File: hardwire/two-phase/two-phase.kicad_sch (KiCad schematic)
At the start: 75 parts, among them Q1 BC847, Q2 IRF3205, Q3 IRF3205, Q4 IRF3205, Q5 IRF3205, U1 74HC244, U2 UC2845_SOIC8, U3 IRS2003, U4 IRS2003, U5 LM7812_TO220, U6 LM7805_TO220

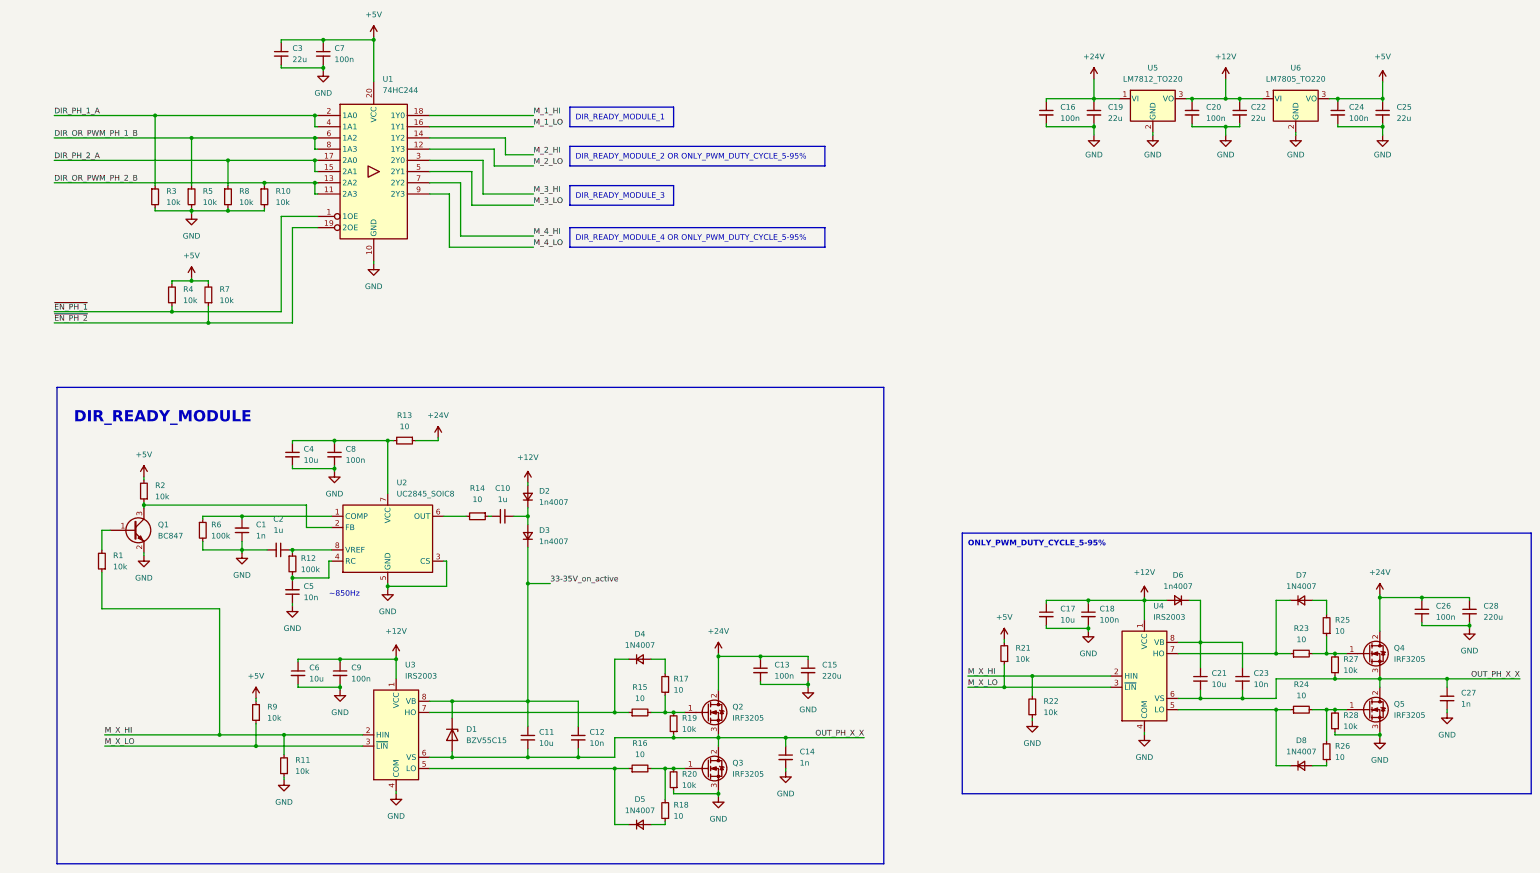
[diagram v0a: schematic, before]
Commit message: hardwire updete
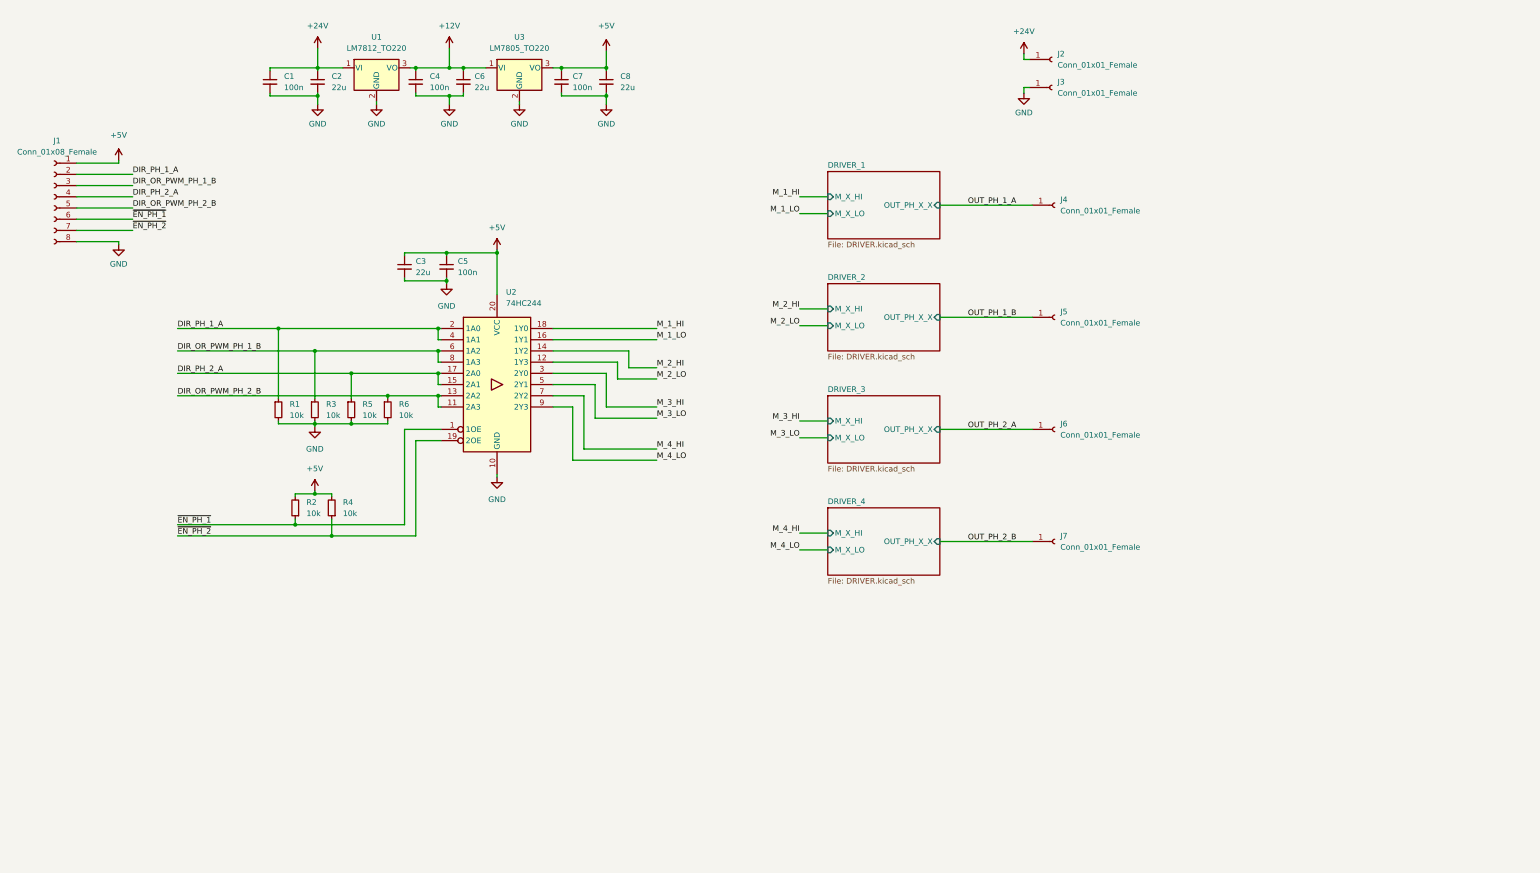
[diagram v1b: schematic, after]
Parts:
- removed C1, C14, C27: 1n, symbol Device:C_Small
- removed C10, C2: 1u, symbol Device:C_Small
- removed C11, C17, C21, C4, C6: 10u, symbol Device:C_Small
- removed C12, C23, C5: 10n, symbol Device:C_Small
- removed C13, C18, C26, C8, C9: 100n, symbol Device:C_Small
- removed C15, C28: 220u, symbol Device:C_Small
- removed D1: BZV55C15, Diode_SMD:D_MiniMELF, symbol Diode:BZV55C15
- removed D2, D3, D6: 1n4007, symbol Device:D_Small
- removed D4, D5, D7, D8: 1N4007, symbol Device:D_Small
- removed Q1: BC847, Package_TO_SOT_SMD:SOT-23, symbol Transistor_BJT:BC847
- removed Q2, Q3, Q4, Q5: IRF3205, Package_TO_SOT_THT:TO-220-3_Vertical, symbol Transistor_FET:IRF3205
- removed R1, R11, R19, R2, R20, R21, R22, R27, R28, R9: 10k, symbol Device:R_Small
- removed R12, R6: 100k, symbol Device:R_Small
- removed R13, R14, R15, R16, R17, R18, R23, R24, R25, R26: 10, symbol Device:R_Small
- removed U2: UC2845_SOIC8, Package_SO:SOIC-8_3.9x4.9mm_P1.27mm, symbol Regulator_Controller:UC3844_SOIC8
- removed U3, U4: IRS2003, symbol Driver_FET:IRS2003
- added J1: Conn_01x08_Female, Connector_PinSocket_2.54mm:PinSocket_1x08_P2.54mm_Vertical, symbol Connector:Conn_01x08_Female
- added J2, J3, J4, J5, J6, J7: Conn_01x01_Female, TestPoint:TestPoint_Loop_D3.80mm_Drill2.8mm, symbol Connector:Conn_01x01_Female
- C1: renamed from C16; footprint (none) -> Capacitor_THT:C_Rect_L7.0mm_W6.0mm_P5.00mm
- C2: renamed from C19; footprint (none) -> Capacitor_THT:C_Radial_D8.0mm_H11.5mm_P3.50mm
- C3: footprint (none) -> Capacitor_THT:C_Radial_D8.0mm_H11.5mm_P3.50mm
- C4: renamed from C20; footprint (none) -> Capacitor_THT:C_Rect_L7.0mm_W6.0mm_P5.00mm
- C5: renamed from C7; footprint (none) -> Capacitor_THT:C_Rect_L7.0mm_W6.0mm_P5.00mm
- C6: renamed from C22; footprint (none) -> Capacitor_THT:C_Radial_D8.0mm_H11.5mm_P3.50mm
- C7: renamed from C24; footprint (none) -> Capacitor_THT:C_Rect_L7.0mm_W6.0mm_P5.00mm
- C8: renamed from C25; footprint (none) -> Capacitor_THT:C_Radial_D8.0mm_H11.5mm_P3.50mm
- R1: renamed from R3; footprint (none) -> Resistor_THT:R_Axial_DIN0204_L3.6mm_D1.6mm_P5.08mm_Horizontal
- R2: renamed from R4; footprint (none) -> Resistor_THT:R_Axial_DIN0204_L3.6mm_D1.6mm_P5.08mm_Horizontal
- R3: renamed from R5; footprint (none) -> Resistor_THT:R_Axial_DIN0204_L3.6mm_D1.6mm_P5.08mm_Horizontal
- R4: renamed from R7; footprint (none) -> Resistor_THT:R_Axial_DIN0204_L3.6mm_D1.6mm_P5.08mm_Horizontal
- R5: renamed from R8; footprint (none) -> Resistor_THT:R_Axial_DIN0204_L3.6mm_D1.6mm_P5.08mm_Horizontal
- R6: renamed from R10; footprint (none) -> Resistor_THT:R_Axial_DIN0204_L3.6mm_D1.6mm_P5.08mm_Horizontal
- U2: renamed from U1; footprint (none) -> Package_DIP:DIP-20_W7.62mm
- renumbered U5 to U1, U6 to U3
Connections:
- net +24V: now also J2.1 (Pin_1)
- net +5V: now also J1.1 (Pin_1)
- net DIR_OR_PWM_PH_1_B: now also J1.3 (Pin_3)
- net DIR_OR_PWM_PH_2_B: now also J1.5 (Pin_5)
- net DIR_PH_1_A: now also J1.2 (Pin_2)
- net DIR_PH_2_A: now also J1.4 (Pin_4)
- net GND: now also J1.8 (Pin_8), J3.1 (Pin_1)
- net ~{EN_PH_1}: now also J1.6 (Pin_6)
- net ~{EN_PH_2}: now also J1.7 (Pin_7)
- new net OUT_PH_1_A: J4.1 (Pin_1)
- new net OUT_PH_1_B: J5.1 (Pin_1)
- new net OUT_PH_2_A: J6.1 (Pin_1)
- new net OUT_PH_2_B: J7.1 (Pin_1)
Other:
- added sheet DRIVER_1 (DRIVER.kicad_sch)
- added sheet DRIVER_2 (DRIVER.kicad_sch)
- added sheet DRIVER_3 (DRIVER.kicad_sch)
- added sheet DRIVER_4 (DRIVER.kicad_sch)
- note removed: "DIR_READY_MODULE"
- note removed: "DIR_READY_MODULE_1"
- note removed: "DIR_READY_MODULE_2 OR ONLY_PWM_DUTY_CYCLE_5-95%"
- note removed: "DIR_READY_MODULE_3"
- note removed: "DIR_READY_MODULE_4 OR ONLY_PWM_DUTY_CYCLE_5-95%"
- note removed: "ONLY_PWM_DUTY_CYCLE_5-95%"
- note removed: "~850Hz"
- moved on the sheet: C1, C2, C3, C4, C5, C6, C7, C8, R1, R2, R3, R4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
